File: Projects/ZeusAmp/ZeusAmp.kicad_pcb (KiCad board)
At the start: 2 copper layers, 147.3 x 116.8 mm, 62 parts, among them Q1 NZT660, Q11 NZT660, Q12 NZT660, Q121 NZT660, Q2 NZT660, Q21 NZT660, Q3 PZTA06, Q31 PZTA06, Q4 MJD340T4, Q41 MJD340T4, Q5 MJD350T4, Q51 MJD350T4, Q6 TIP31A, Q61 TIP31A, Q7 PZTA06, Q71 PZTA06, Q8 TIP32C, Q81 TIP32C, Q9 PZTA06, Q91 PZTA06

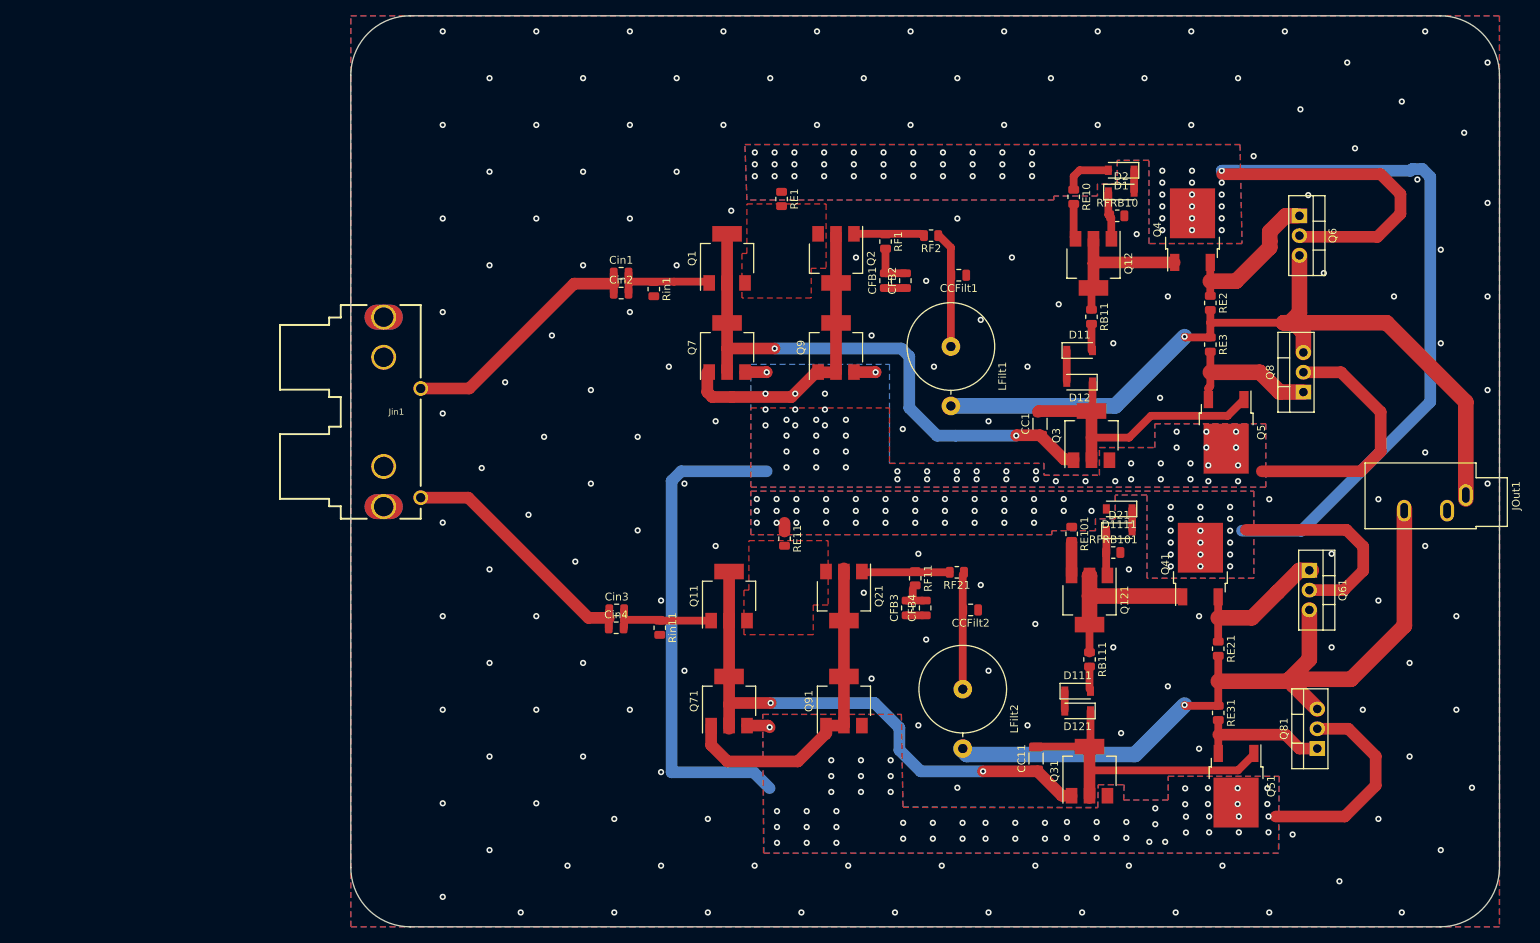
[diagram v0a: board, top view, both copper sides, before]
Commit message: First Zeus V1 completed
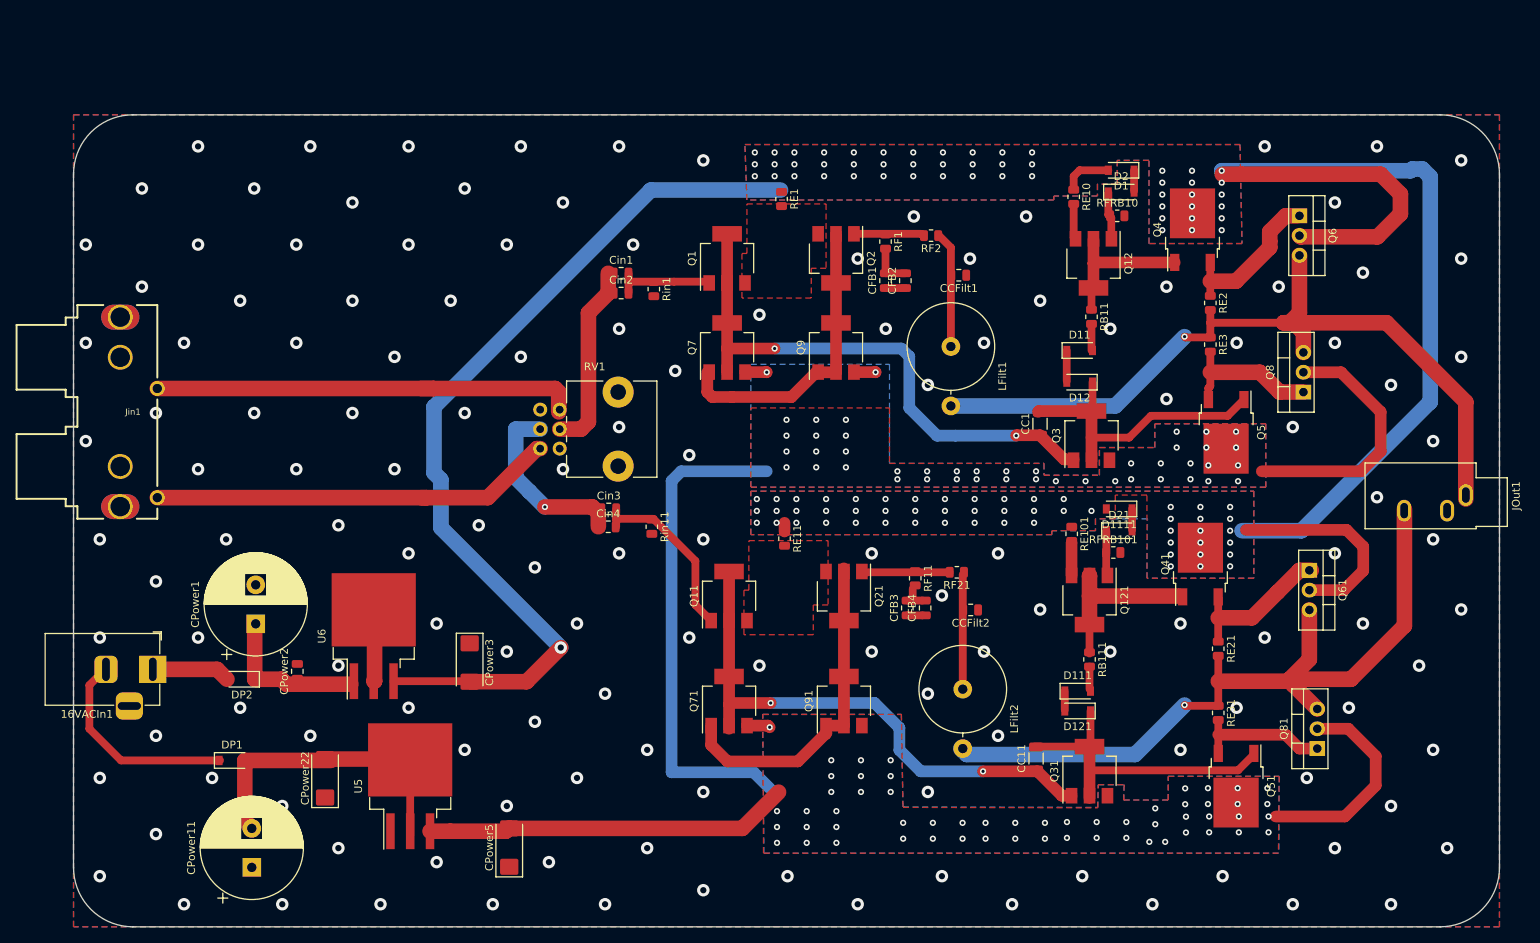
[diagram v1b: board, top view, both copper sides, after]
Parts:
- added 16VACIn1: Barrel_Jack, Connector_BarrelJack:BarrelJack_Horizontal, F.Cu at (33.0, 134.6)
- added CPower1: 1000u, Capacitor_THT:CP_Radial_D13.0mm_P5.00mm, F.Cu at (46.2, 128.8)
- added CPower11: 1000u, Capacitor_THT:CP_Radial_D13.0mm_P5.00mm, F.Cu at (45.7, 160.0)
- added CPower2: 10u, Capacitor_SMD:C_0805_2012Metric, F.Cu at (51.6, 134.9)
- added CPower22: 10u, Capacitor_Tantalum_SMD:CP_EIA-6032-28_Kemet-C, F.Cu at (55.1, 148.6)
- added CPower3: 10u, Capacitor_Tantalum_SMD:CP_EIA-6032-28_Kemet-C, F.Cu at (73.7, 133.7)
- added CPower5: 10u, Capacitor_Tantalum_SMD:CP_EIA-6032-28_Kemet-C, F.Cu at (78.7, 157.5)
- added DP1: 1N4148W, Diode_SMD:D_SOD-123, F.Cu at (43.2, 146.3)
- added DP2: 1N4148W, Diode_SMD:D_SOD-123, F.Cu at (44.5, 135.9)
- added RV1: R_POT_Dual, Potentiometer_THT:Potentiometer_Alps_RK09L_Double_Vertical, F.Cu at (85.2, 106.3)
- added U5: LM2990S-15_NOPB, Package_TO_SOT_SMD:TO-263-3_TabPin2, F.Cu at (66.0, 149.6)
- added U6: LM2937ESX-15_NOPB, Package_TO_SOT_SMD:TO-263-3_TabPin2, F.Cu at (61.4, 130.4)
- moved Jin1 33.8 mm to (30.5, 101.6)
- moved Cin4 13.0 mm to (91.4, 116.3)
- moved Rin11 13.0 mm to (97.0, 116.3)
- moved Cin3 13.0 mm to (91.5, 114.0)
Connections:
- Jin1 pad 2: Net-(Cin1-Pad1) -> Net-(Jin1-Pad2)
- Jin1 pad 4: Net-(Cin3-Pad1) -> Net-(Jin1-Pad4)
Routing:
- net /VCC: track 164.3 -> 281.6 mm, vias 105 -> 106
- net Net-(Jin1-Pad2): track 0.00 -> 55.9 mm
- net Net-(Jin1-Pad4): track 0.00 -> 52.5 mm
- net /VEE: track 132.6 -> 179.5 mm
- net Net-(CPower11-Pad2): track 0.00 -> 40.6 mm
- net /V-: track 0.00 -> 27.0 mm
- net Net-(CPower1-Pad1): track 0.00 -> 19.7 mm
- net /V+: track 0.00 -> 10.1 mm
- net Net-(Cin3-Pad2): track 13.4 -> 23.2 mm
- net Net-(Cin3-Pad1): track 32.6 -> 23.6 mm, vias 0 -> 1
- net GND: track 4.50 -> 13.5 mm, vias 159 -> 143
- net Net-(Cin1-Pad1): track 32.8 -> 24.2 mm
- net Net-(Q2-Pad2): vias 2 -> 0
- net (no net): vias 7 -> 0
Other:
- board size 147.3 x 116.8 mm -> 182.9 x 104.1 mm
